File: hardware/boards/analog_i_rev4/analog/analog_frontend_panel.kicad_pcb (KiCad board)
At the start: 4 copper layers, 257 parts, among them IC1 INA826AIDR, IC10 INA826AIDR, IC1001 INA826AIDR, IC12 INA826AIDR, IC13 TLV333IDBVR, IC14 TLV333IDBVR, IC15 INA826AIDR, IC16 TLV333IDBVR, IC17 TLV333IDBVR, IC18 INA826AIDR, IC19 TLV333IDBVR, IC2 INA826AIDR, IC20 TLV333IDBVR, IC21 INA826AIDR, IC22 TLV333IDBVR, IC23 TLV333IDBVR, IC24 INA826AIDR, IC25 TLV333IDBVR, IC26 TLV333IDBVR, IC27 INA826AIDR, IC28 TLV333IDBVR, IC29 TLV333IDBVR, IC3 INA826AIDR, IC3001 INA826AIDR, IC3002 INA826AIDR, IC32001 BD42540FJ-CE2, IC33001 BD42540FJ-CE2, IC34001 BD42540FJ-CE2, IC35001 BD42540FJ-CE2, IC36001 BD42540FJ-CE2, IC4 INA826AIDR, IC5 INA826AIDR, IC6 INA826AIDR, IC7 INA826AIDR, IC8 INA826AIDR, J10 Screw_Terminal_01x03, J1001 Screw_Terminal_01x04, J11 Screw_Terminal_01x03, J12 AM-K-PCB, J13 AM-K-PCB, J14 AM-K-PCB, J15 AM-K-PCB, J16 Screw_Terminal_01x03, J17 Screw_Terminal_01x03, J18 Screw_Terminal_01x03, J19 Screw_Terminal_01x03, J20 Screw_Terminal_01x03, J22 Screw_Terminal_01x03, J3 Screw_Terminal_01x04, J3004 Screw_Terminal_01x04, J3005 Screw_Terminal_01x04, J4 Screw_Terminal_01x04, J5 Screw_Terminal_01x04, J8 Screw_Terminal_01x03, J9 Screw_Terminal_01x03, U1 NTJD4001NT1G, U1001 TLV3201AIDBVR, U1002 TLV3201AIDBVR, U1003 TLV3201AIDBVR, U1004 TLV3201AIDBVR, U1005 TLV3201AIDBVR, U2 NTJD4001NT1G, U3 NTJD4001NT1G, U4 NTJD4001NT1G, U5 NTJD4001NT1G, U6 NTJD4001NT1G

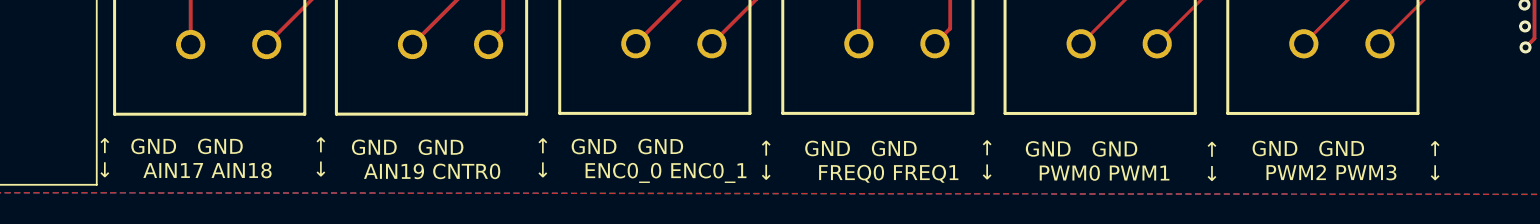
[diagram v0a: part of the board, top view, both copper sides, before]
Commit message: update combined project
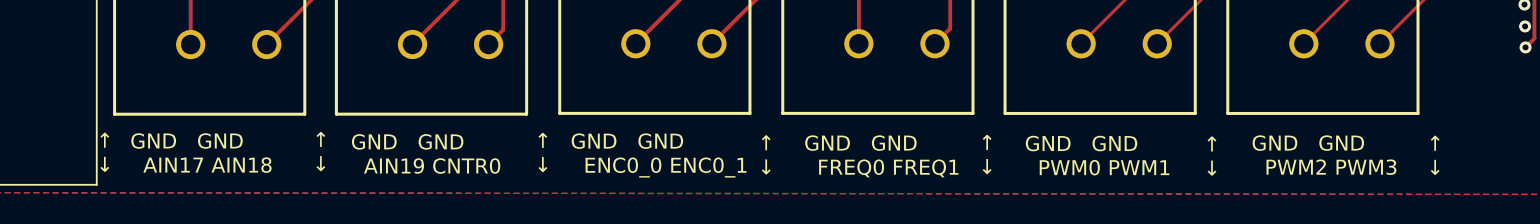
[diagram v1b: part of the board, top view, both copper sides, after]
